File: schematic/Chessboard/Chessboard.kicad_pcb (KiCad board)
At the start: 2 copper layers, 29 parts, among them J1 LED, J2 VOUT, J3 Data, J4 VOUT, J5 Data, Q1 BC640, Q2 BC640, Q3 BC640, Q4 BC640, Q5 BC640, Q6 BC640, Q7 BC640, Q8 BC640, SW1 SW_SPST, U1 Logic Level Shifter, U2 Batterie Shield, U3 Logic Level Shifter, U4 Logic Level Shifter, U5 Logic Level Shifter

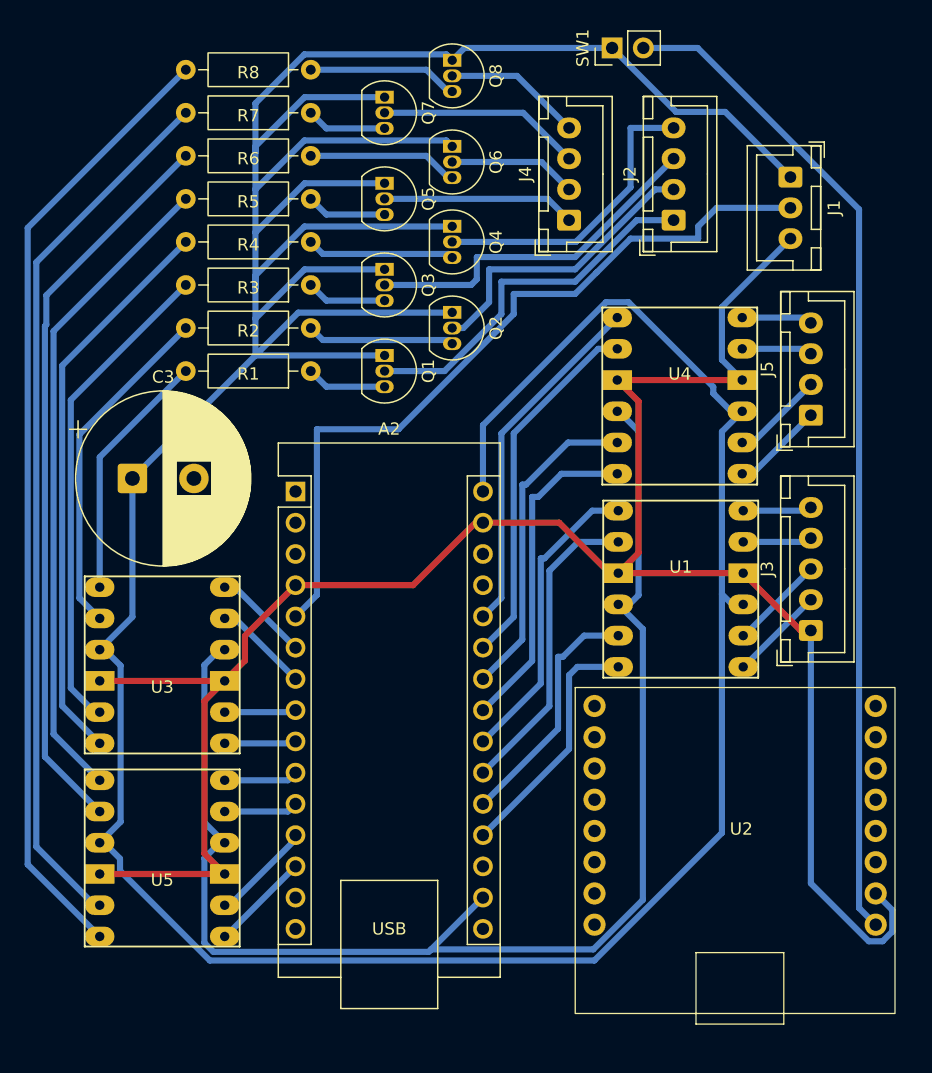
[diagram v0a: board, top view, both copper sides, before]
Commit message: finish Mainboard design
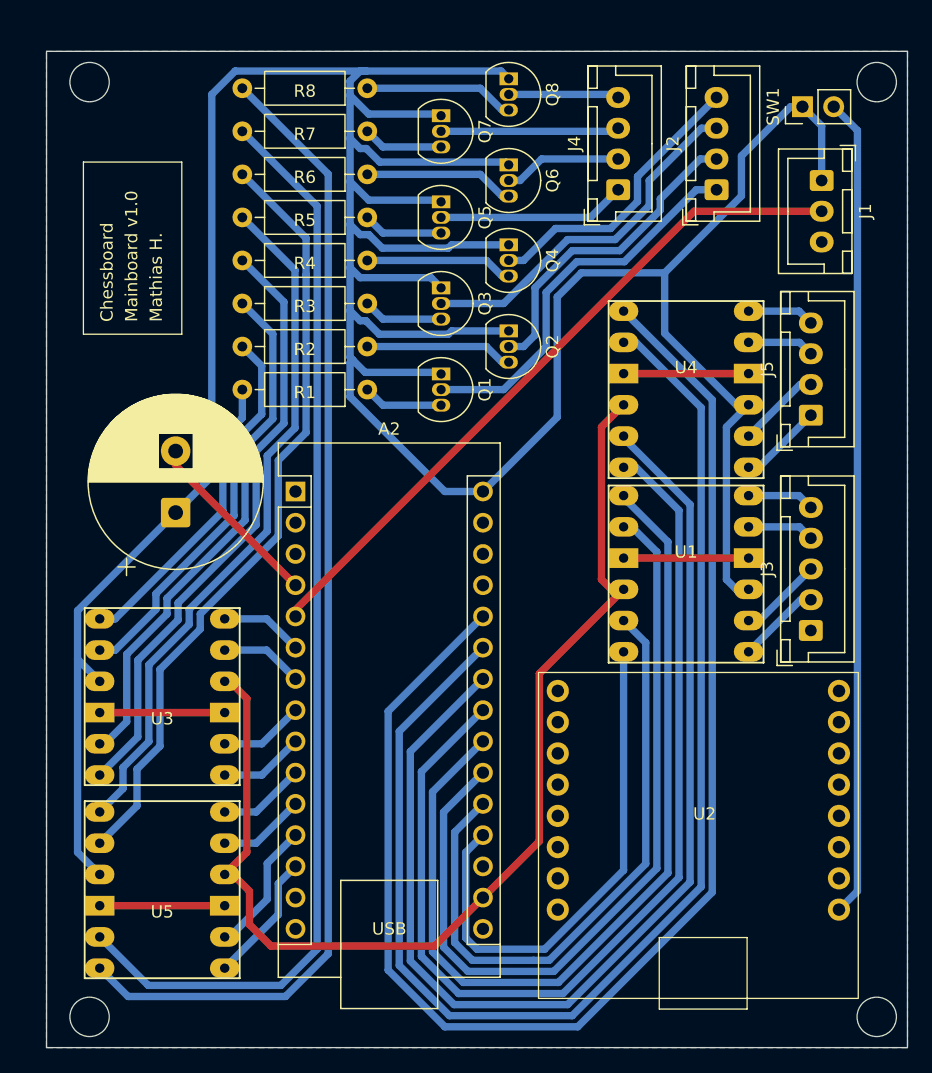
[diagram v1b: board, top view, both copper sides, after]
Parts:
- added ?: , , F.Cu at (113.0, 118.5)
- added ?: , , F.Cu at (177.0, 42.5)
- added ?: , , F.Cu at (113.0, 42.5)
- added REF**: MountingHole_3.2mm_M3, MountingHole:MountingHole_3.2mm_M3, F.Cu at (177.0, 118.5)
- moved SW1 16.2 mm to (171.0, 44.5)
- moved Q1 4.84 mm to (141.6, 66.2)
- moved R1 4.84 mm to (135.6, 67.5)
- moved R2 4.84 mm to (135.6, 64.0)
- moved R3 4.84 mm to (135.6, 60.5)
- moved R4 4.84 mm to (135.6, 57.0)
- moved R5 4.84 mm to (135.6, 53.5)
- moved R6 4.84 mm to (135.6, 50.0)
- moved R7 4.84 mm to (135.6, 46.5)
- moved R8 4.84 mm to (135.6, 43.0)
- moved Q2 4.84 mm to (147.1, 62.7)
- moved Q3 4.84 mm to (141.6, 59.2)
- moved Q4 4.84 mm to (147.1, 55.7)
- moved Q5 4.84 mm to (141.6, 52.2)
- moved Q6 4.84 mm to (147.1, 49.2)
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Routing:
- net GND: track 170.1 -> 55.6 mm
- net Net-(A2-A7): track 28.8 -> 115.0 mm
- net Net-(A2-A6): track 29.7 -> 106.7 mm
- net Net-(A2-SCL/A5): track 26.3 -> 92.2 mm
- net Net-(A2-SDA/A4): track 26.7 -> 84.0 mm
- net +5V: track 350.1 -> 295.7 mm
- net Net-(A2-A3): track 24.7 -> 74.8 mm
- net Net-(A2-A2): track 25.2 -> 66.4 mm
- net Net-(A2-A1): track 20.1 -> 52.1 mm
- net Net-(A2-A0): track 20.2 -> 42.6 mm
- net +3V3: track 112.6 -> 90.9 mm
- net Net-(U5-HV3): track 71.8 -> 89.5 mm
- net Net-(U5-HV4): track 78.2 -> 94.2 mm
- net Net-(SW1-B): track 81.7 -> 66.7 mm
- net /LED_ROW_1_2/LED_Data: track 63.4 -> 56.7 mm
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- added copper zone on B.Cu, net GND
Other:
- board outline added: 70 x 81 mm
- board text added: "Chessboard"
- board text added: "Mainboard v1.0"
- board text added: "Mathias H."
